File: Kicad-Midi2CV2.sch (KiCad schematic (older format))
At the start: 119 parts, among them IC101 MCP4725module, IC102 MCP4725module, J101 Doepfer connector, J102 Vin 7-12v, J103 MIDI OUT, J104 Power Conn, J105 CV7 in, J106 Gate1, J107 MIDI IN, J108 CV6 in, J109 Gate2, J110 CV3 in, J111 Gate3, J112 CV1, J113 Gate4, J114 CV2, J115 ControlConn, J116 ControlConn, J117 I2C_Conn, J118 I2C_Conn, Q101 MMBT2222A, Q102 MMBT2222A, SW101 Rotary_Encoder_Switch, U101 TL072, U102 TL072, U103 EL814

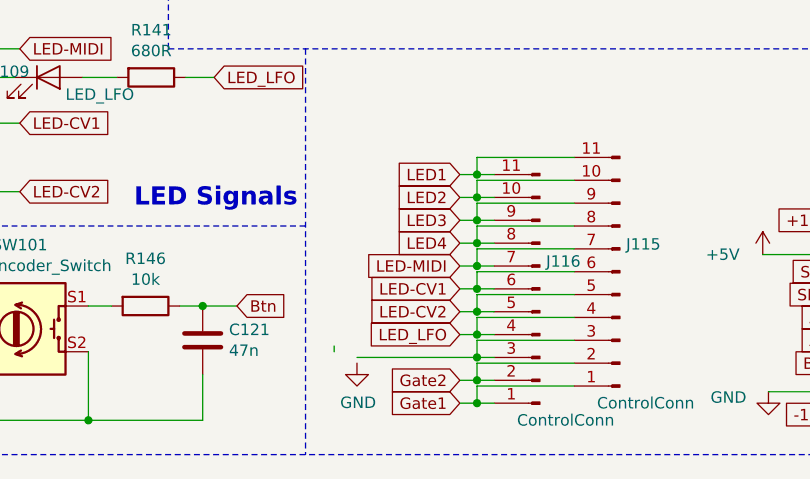
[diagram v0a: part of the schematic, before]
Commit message: Routing....
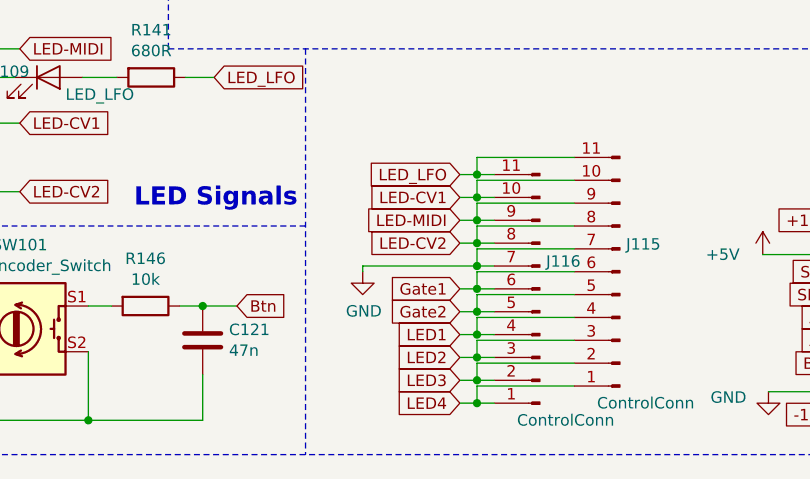
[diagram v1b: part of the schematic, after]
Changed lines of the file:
@@
 Text GLabel 2400 5975 2    50   Input ~ 0
 LED-MIDI
-Text GLabel 4325 6525 0    50   Input ~ 0
+Text GLabel 4325 7225 0    50   Input ~ 0
 LED1
-Text GLabel 4325 6625 0    50   Input ~ 0
+Text GLabel 4325 7325 0    50   Input ~ 0
 LED2
-Text GLabel 4325 6725 0    50   Input ~ 0
+Text GLabel 4325 7425 0    50   Input ~ 0
 LED3
-Text GLabel 4325 6825 0    50   Input ~ 0
+Text GLabel 4325 7525 0    50   Input ~ 0
 LED4
 $Comp
@@
 Wire Wire Line
 	1150 7600 1300 7600
-Text GLabel 4325 7525 0    50   Input ~ 0
+Text GLabel 4325 7025 0    50   Input ~ 0
 Gate1
-Text GLabel 4325 7425 0    50   Input ~ 0
+Text GLabel 4325 7125 0    50   Input ~ 0
 Gate2
 Text GLabel 5350 4800 2    50   Input ~ 0
@@
 Wire Notes Line
 	6300 500  8525 500
-Text GLabel 4325 7125 0    50   Input ~ 0
+Text GLabel 4325 6825 0    50   Input ~ 0
 LED-CV2
-Text GLabel 4325 7025 0    50   Input ~ 0
+Text GLabel 4325 6625 0    50   Input ~ 0
 LED-CV1
-Text GLabel 4325 6925 0    50   Input ~ 0
+Text GLabel 4325 6725 0    50   Input ~ 0
 LED-MIDI
 Wire Notes Line
@@
 L power:GND #PWR0128
 U 1 1 5CAA25A2
-P 3875 7350
-F 0 "#PWR0128" H 3875 7100 50  0001 C CNN
-F 1 "GND" H 3880 7177 50  0000 C CNN
-F 2 "" H 3875 7350 50  0001 C CNN
-F 3 "" H 3875 7350 50  0001 C CNN
-	1    3875 7350
+P 3900 6950
+F 0 "#PWR0128" H 3900 6700 50  0001 C CNN
+F 1 "GND" H 3905 6777 50  0000 C CNN
+F 2 "" H 3900 6950 50  0001 C CNN
+F 3 "" H 3900 6950 50  0001 C CNN
+	1    3900 6950
 	1    0    0    -1
 $EndComp
@@
 	4325 6825 4400 6825
 Wire Wire Line
-	4325 6925 4400 6925
-Wire Wire Line
 	4325 7025 4400 7025
 Wire Wire Line
@@
 Wire Wire Line
 	4325 7425 4400 7425
-Wire Wire Line
-	3775 7275 3775 7300
 Wire Wire Line
 	4475 7225 4400 7225
@@
 Wire Wire Line
 	4400 7250 4400 7325
-Connection ~ 4400 7325
 Wire Wire Line
 	4400 7325 4475 7325
@@
 Wire Wire Line
 	2575 900  3050 900
-Text GLabel 4325 7225 0    50   Input ~ 0
+Text GLabel 4325 6525 0    50   Input ~ 0
 LED_LFO
 Wire Wire Line
@@
 Connection ~ 6000 7475
 Wire Wire Line
-	3875 7325 4400 7325
-Wire Wire Line
 	4325 7525 4400 7525
 Connection ~ 4400 7525
@@
 $EndComp
 $Comp
-L power:GND #PWR?
+L power:GND #PWR0131
 U 1 1 5D3B40A8
 P 7850 5000
-F 0 "#PWR?" H 7850 4750 50  0001 C CNN
+F 0 "#PWR0131" H 7850 4750 50  0001 C CNN
 F 1 "GND" H 7855 4827 50  0000 C CNN
 F 2 "" H 7850 5000 50  0001 C CNN
@@
 	1    0    0    -1
 $EndComp
+Wire Wire Line
+	3900 6925 3900 6950
+Wire Wire Line
+	3900 6925 4400 6925
+Wire Wire Line
+	4325 7325 4400 7325
+Connection ~ 4400 7325
 $EndSCHEMATC
